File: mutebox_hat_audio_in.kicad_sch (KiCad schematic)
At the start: 23 parts, among them J1 GPIO, U1 CAT24C256, U2 74LVC157, U3 PCM1862DBT

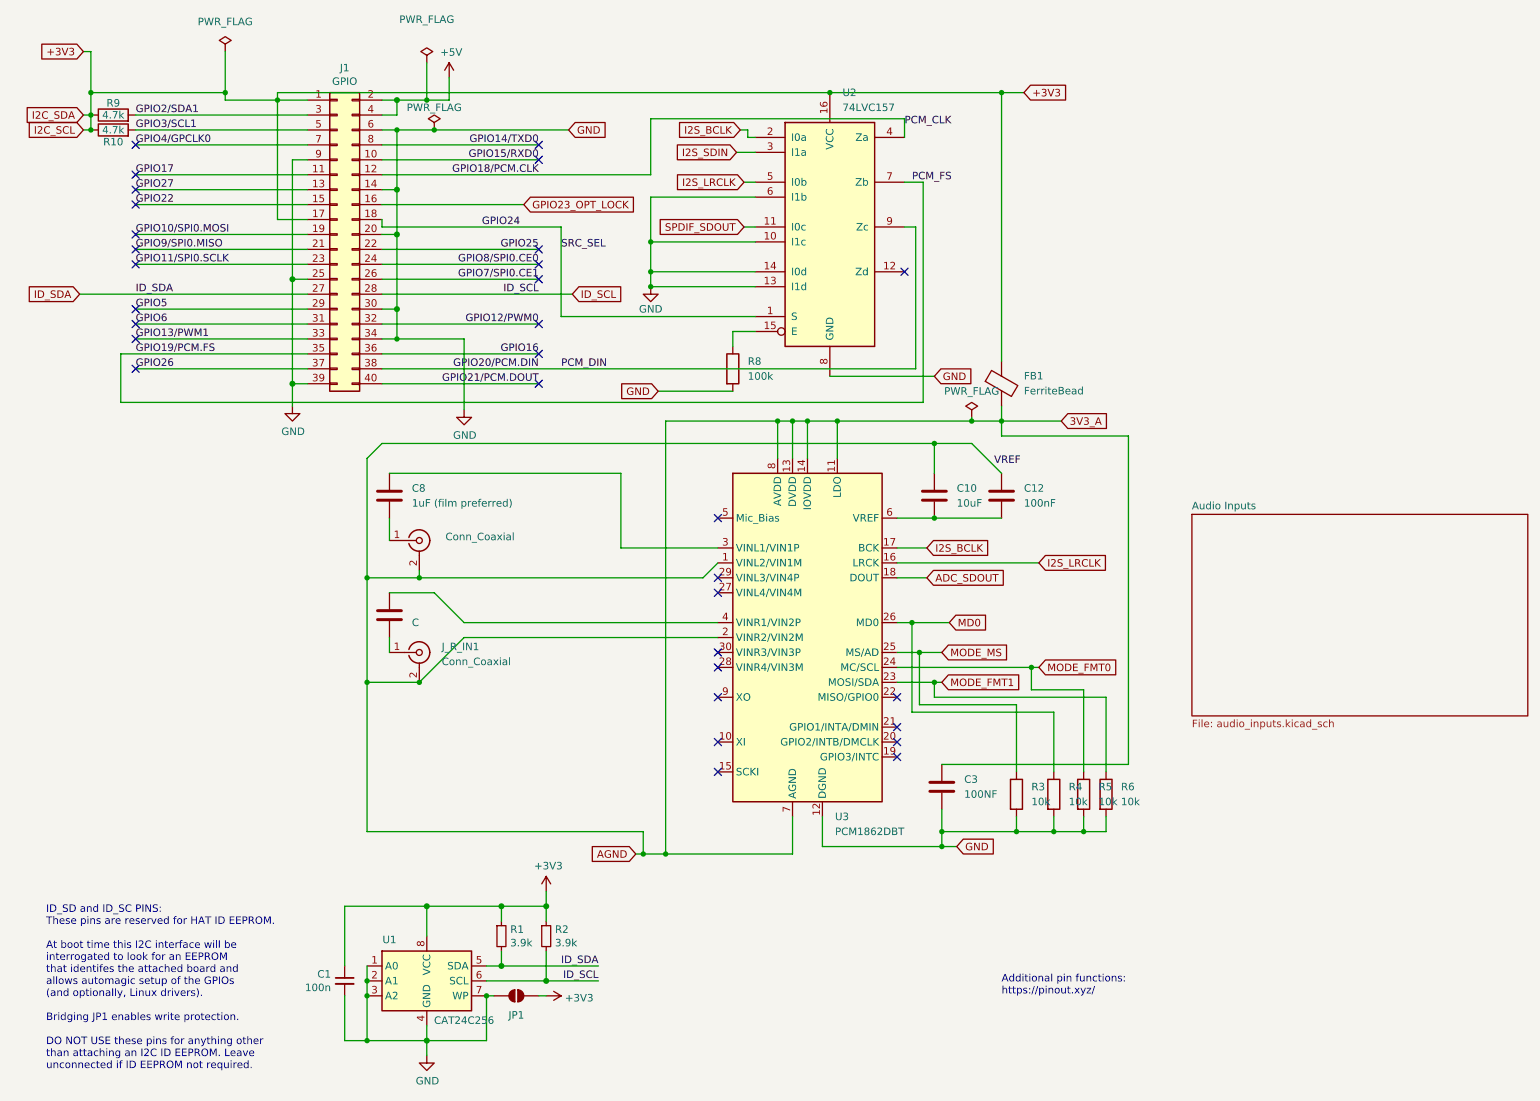
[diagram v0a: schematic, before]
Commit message: Fixed some connections and global labels
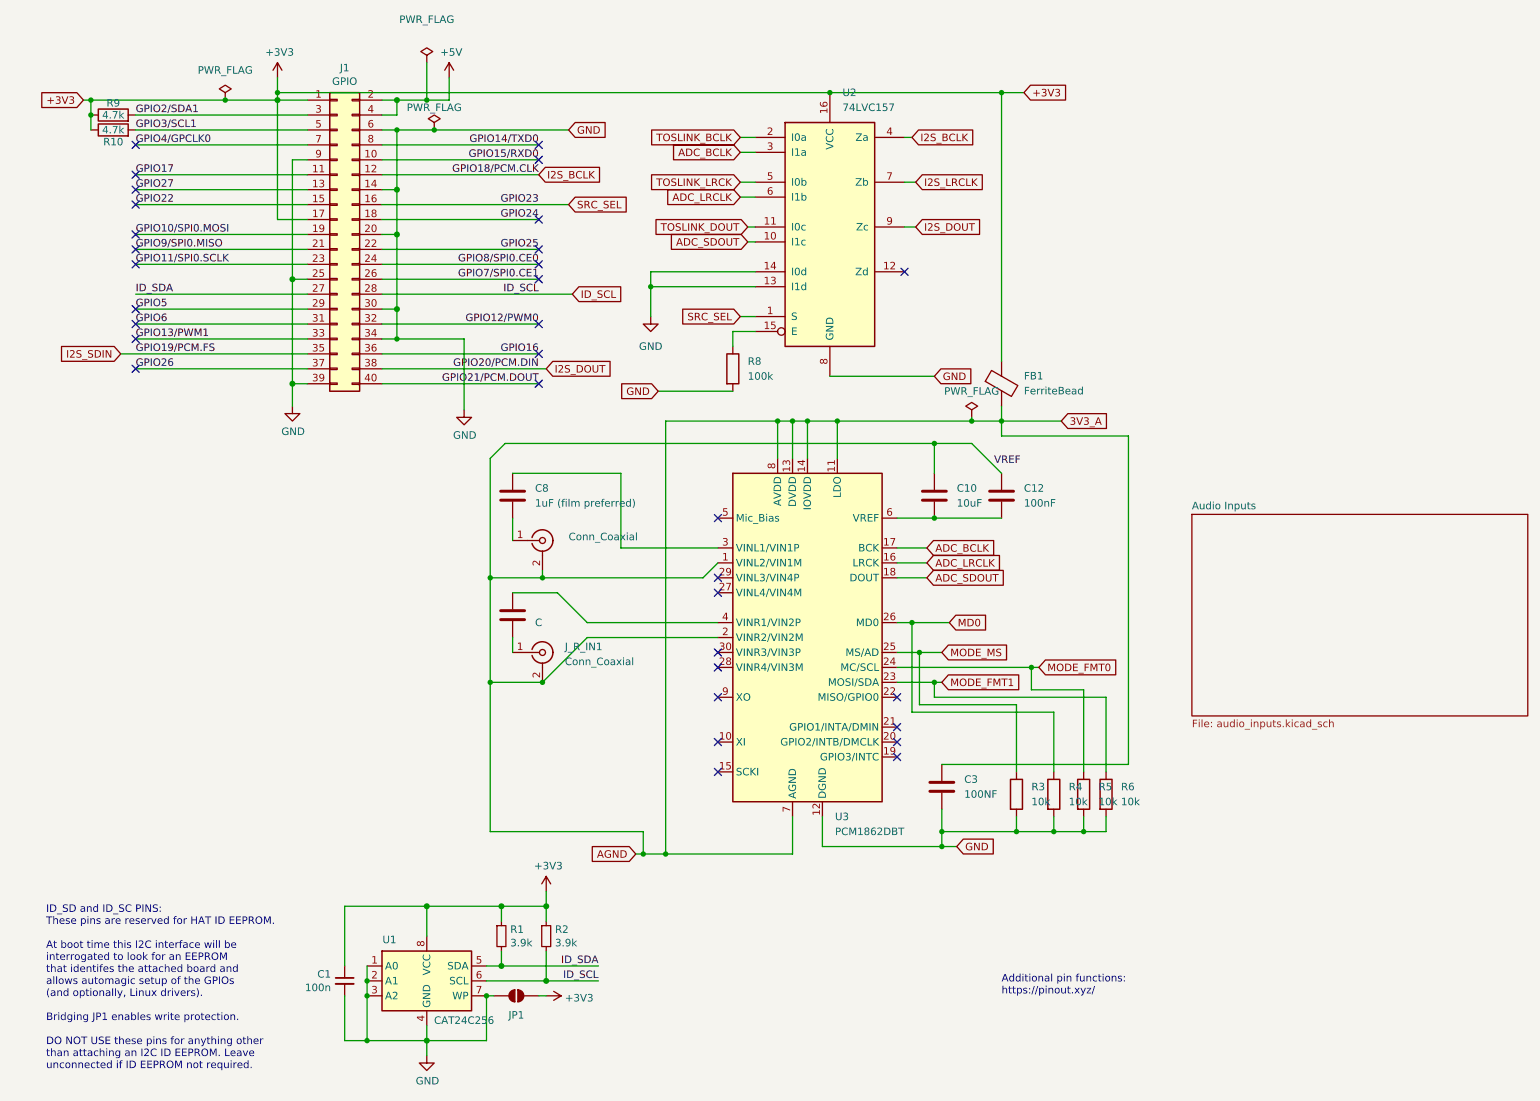
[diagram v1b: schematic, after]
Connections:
- net GPIO18/PCM.CLK is gone; now on net I2S_BCLK: J1.12 (Pin_12), U2.4 (Za)
- net ADC_SDOUT: now also U2.10 (I1c)
- net GND: no longer U2.10 (I1c), U2.6 (I1b)
- net GPIO24: no longer U2.1 (S)
- net I2S_BCLK: no longer U2.2 (I0a), U3.17 (BCK)
- net I2S_LRCLK: now also U2.7 (Zb); no longer U2.5 (I0b), U3.16 (LRCK)
- net I2S_SDIN: now also J1.35 (Pin_35); no longer U2.3 (I1a)
- removed net GPIO19/PCM.FS: J1.35 (Pin_35), U2.7 (Zb)
- net GPIO20/PCM.DIN renamed I2S_DOUT
- net GPIO23_OPT_LOCK renamed SRC_SEL
- net SRC_SEL: now also U2.1 (S)
- net SPDIF_SDOUT renamed TOSLINK_DOUT
- new net ADC_BCLK: U2.3 (I1a), U3.17 (BCK)
- new net ADC_LRCLK: U2.6 (I1b), U3.16 (LRCK)
- new net TOSLINK_BCLK: U2.2 (I0a)
- new net TOSLINK_LRCK: U2.5 (I0b)
- no-connect marks 32 -> 33
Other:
- moved on the sheet: C8, J_R_IN1
